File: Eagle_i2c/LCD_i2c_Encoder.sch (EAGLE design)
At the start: 8 parts, among them J1 455-1750-1-ND, U1 ARDUINOR3-BPLACE

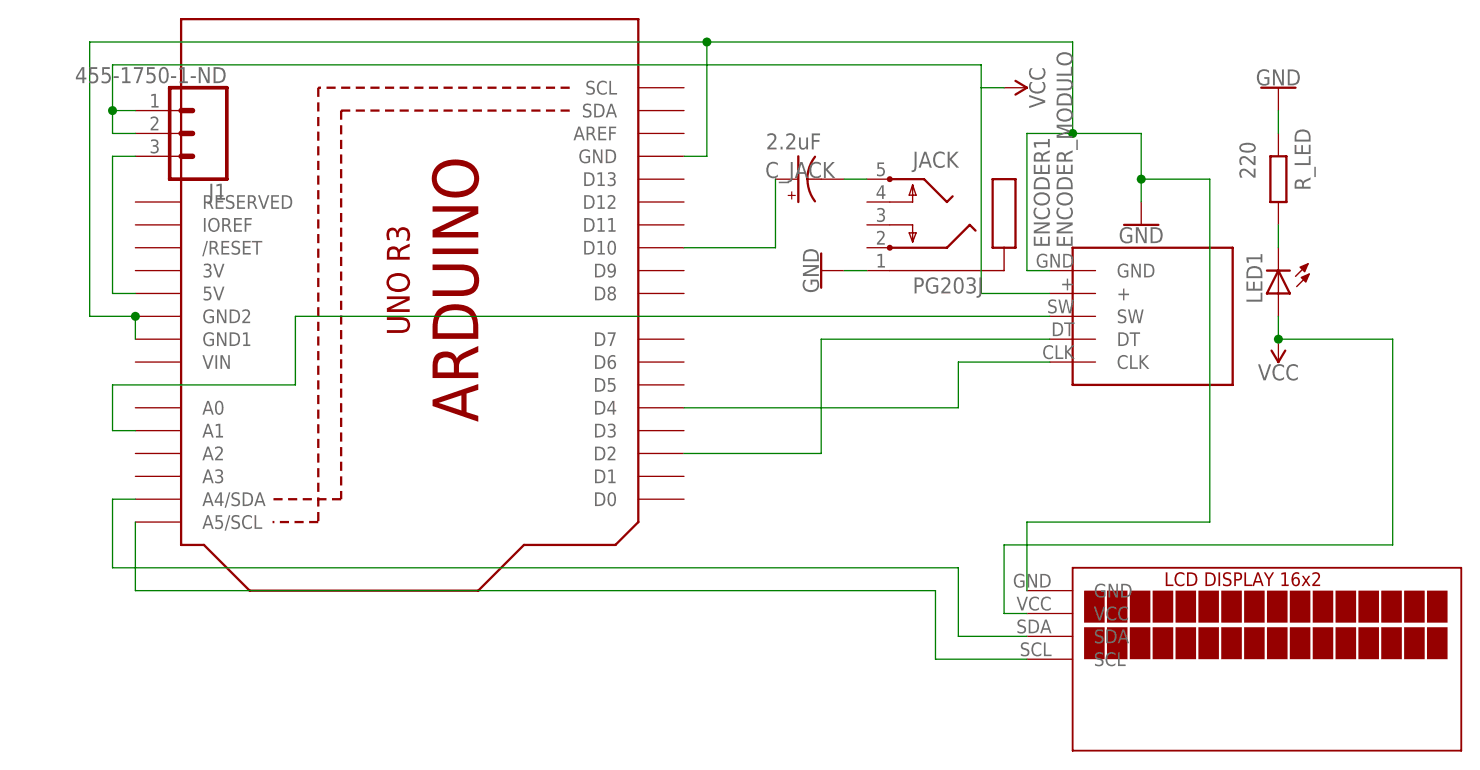
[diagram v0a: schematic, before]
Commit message: Version para imprimir ICAT, Gerbers incluidos
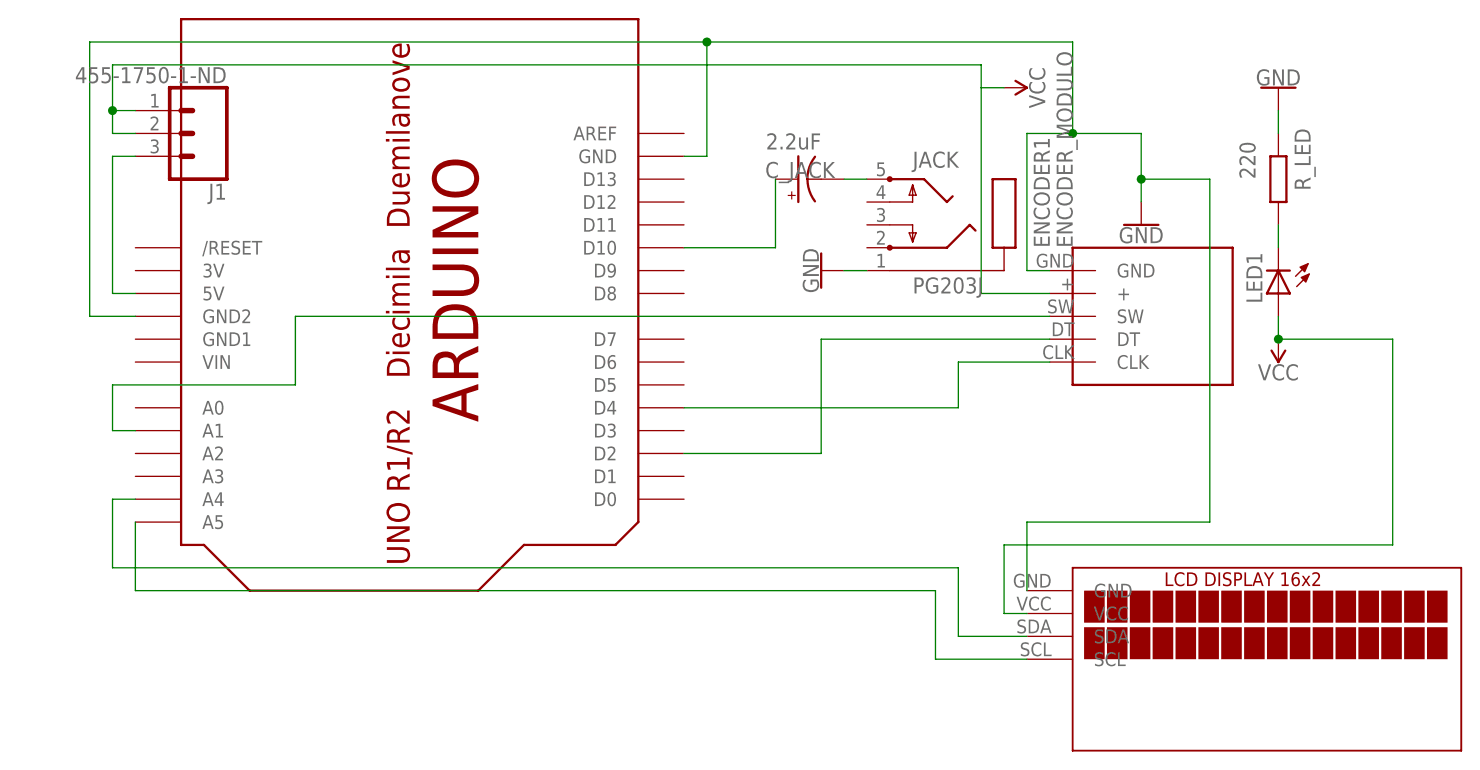
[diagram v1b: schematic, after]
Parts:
- removed U1: ARDUINOR3-BPLACE, adafruit:ARDUINOR3-BPLACE
- added U$1: ARDUINOUNO, Arduino_Espejo:ARDUINOUNO
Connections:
- net GND: now also U$1.GND, U$1.GND2; no longer U1.GND, U1.GND1, U1.GND2
- net N$1: now also U$1.D10; no longer U1.D10
- net N$17: now also U$1.D4; no longer U1.D4
- net N$18: now also U$1.D2; no longer U1.D2
- net N$3: now also U$1.A1; no longer U1.A1
- net N$5: now also U$1.5V; no longer U1.5V
- net N$8: now also U$1.A4; no longer U1.A4/SDA
- net N$9: now also U$1.A5; no longer U1.A5/SCL
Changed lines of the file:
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@@
 </variantdefs>
 <classes>
-<class number="0" name="default" width="0.3" drill="0.0127">
-<clearance class="0" value="0.3"/>
+<class number="0" name="default" width="0.3048" drill="0.3048">
+<clearance class="0" value="0.3048"/>
 </class>
 </classes>
@@
 <attribute name="CAPACITANCIA" value="2.2uF"/>
 </part>
-<part name="U1" library="adafruit" deviceset="ARDUINOR3" device="-BPLACE"/>
 <part name="SUPPLY1" library="SparkFun-PowerSymbols" deviceset="VCC" device=""/>
 <part name="SUPPLY2" library="SparkFun-PowerSymbols" deviceset="VCC" device=""/>
@@
 <part name="ENCODER1" library="ENCODER" deviceset="ENCODER_MODULO" device=""/>
 <part name="J1" library="SparkFun-Connectors" deviceset="CONN_03" device="" value="455-1750-1-ND"/>
+<part name="U$1" library="Arduino_Espejo" deviceset="ARDUINO" device="UNO"/>
 </parts>
 <sheets>
@@
 <attribute name="CAPACITANCIA" x="71.12" y="81.28" size="1.778" layer="96" rot="R180"/>
 </instance>
-<instance part="U1" gate="G$1" x="25.4" y="60.96" smashed="yes" rot="R270"/>
 <instance part="SUPPLY1" gate="G$1" x="91.44" y="86.36" smashed="yes" rot="R270">
 <attribute name="VALUE" x="94.234" y="86.36" size="1.778" layer="96" rot="R270" align="bottom-center"/>
@@
 <attribute name="NAME" x="5.08" y="75.692" size="1.778" layer="95" font="vector" rot="R180"/>
 </instance>
+<instance part="U$1" gate="G$1" x="27.94" y="71.12" smashed="yes" rot="R270"/>
 </instances>
 <busses>
@@
 <wire x1="99.06" y1="81.28" x2="106.68" y2="81.28" width="0.1524" layer="91"/>
 <wire x1="106.68" y1="81.28" x2="106.68" y2="76.2" width="0.1524" layer="91"/>
-<pinref part="U1" gate="G$1" pin="GND2"/>
 <wire x1="106.68" y1="76.2" x2="106.68" y2="73.66" width="0.1524" layer="91"/>
-<wire x1="-5.08" y1="60.96" x2="-10.16" y2="60.96" width="0.1524" layer="91"/>
 <wire x1="-10.16" y1="60.96" x2="-10.16" y2="91.44" width="0.1524" layer="91"/>
 <wire x1="-10.16" y1="91.44" x2="58.42" y2="91.44" width="0.1524" layer="91"/>
@@
 <wire x1="99.06" y1="91.44" x2="99.06" y2="81.28" width="0.1524" layer="91"/>
 <junction x="99.06" y="81.28"/>
-<pinref part="U1" gate="G$1" pin="GND1"/>
-<wire x1="-5.08" y1="58.42" x2="-5.08" y2="60.96" width="0.1524" layer="91"/>
-<junction x="-5.08" y="60.96"/>
-<pinref part="U1" gate="G$1" pin="GND"/>
-<wire x1="55.88" y1="78.74" x2="58.42" y2="78.74" width="0.1524" layer="91"/>
 <wire x1="58.42" y1="78.74" x2="58.42" y2="91.44" width="0.1524" layer="91"/>
 <junction x="58.42" y="91.44"/>
@@
 <pinref part="ENCODER1" gate="G$1" pin="GND"/>
 <wire x1="93.98" y1="66.04" x2="96.52" y2="66.04" width="0.1524" layer="91"/>
+<wire x1="-10.16" y1="60.96" x2="-5.08" y2="60.96" width="0.1524" layer="91"/>
+<wire x1="55.88" y1="78.74" x2="58.42" y2="78.74" width="0.1524" layer="91"/>
+<pinref part="U$1" gate="G$1" pin="GND"/>
+<pinref part="U$1" gate="G$1" pin="GND2"/>
 </segment>
 <segment>
@@
 <segment>
 <wire x1="86.36" y1="55.88" x2="86.36" y2="50.8" width="0.1524" layer="91"/>
-<pinref part="U1" gate="G$1" pin="D4"/>
-<wire x1="55.88" y1="50.8" x2="86.36" y2="50.8" width="0.1524" layer="91"/>
 <wire x1="86.36" y1="55.88" x2="96.52" y2="55.88" width="0.1524" layer="91"/>
 <pinref part="ENCODER1" gate="G$1" pin="CLK"/>
+<wire x1="86.36" y1="50.8" x2="55.88" y2="50.8" width="0.1524" layer="91"/>
+<pinref part="U$1" gate="G$1" pin="D4"/>
 </segment>
 </net>
@@
 <wire x1="71.12" y1="45.72" x2="71.12" y2="58.42" width="0.1524" layer="91"/>
 <wire x1="71.12" y1="58.42" x2="96.52" y2="58.42" width="0.1524" layer="91"/>
-<pinref part="U1" gate="G$1" pin="D2"/>
-<wire x1="55.88" y1="45.72" x2="71.12" y2="45.72" width="0.1524" layer="91"/>
 <pinref part="ENCODER1" gate="G$1" pin="DT"/>
+<wire x1="71.12" y1="45.72" x2="55.88" y2="45.72" width="0.1524" layer="91"/>
+<pinref part="U$1" gate="G$1" pin="D2"/>
 </segment>
 </net>
@@
 <segment>
 <wire x1="96.52" y1="60.96" x2="12.7" y2="60.96" width="0.1524" layer="91"/>
-<pinref part="U1" gate="G$1" pin="A1"/>
-<wire x1="-5.08" y1="48.26" x2="-7.62" y2="48.26" width="0.1524" layer="91"/>
 <wire x1="-7.62" y1="48.26" x2="-7.62" y2="53.34" width="0.1524" layer="91"/>
 <wire x1="-7.62" y1="53.34" x2="12.7" y2="53.34" width="0.1524" layer="91"/>
 <wire x1="12.7" y1="53.34" x2="12.7" y2="60.96" width="0.1524" layer="91"/>
 <pinref part="ENCODER1" gate="G$1" pin="SW"/>
+<wire x1="-5.08" y1="48.26" x2="-7.62" y2="48.26" width="0.1524" layer="91"/>
+<pinref part="U$1" gate="G$1" pin="A1"/>
 </segment>
 </net>
@@
 <pinref part="C_JACK" gate="G$1" pin="+"/>
 <wire x1="66.04" y1="76.2" x2="66.04" y2="68.58" width="0.1524" layer="91"/>
-<pinref part="U1" gate="G$1" pin="D10"/>
-<wire x1="66.04" y1="68.58" x2="55.88" y2="68.58" width="0.1524" layer="91"/>
+<wire x1="55.88" y1="68.58" x2="66.04" y2="68.58" width="0.1524" layer="91"/>
+<pinref part="U$1" gate="G$1" pin="D10"/>
 </segment>
 </net>
 <net name="N$5" class="0">
 <segment>
-<pinref part="U1" gate="G$1" pin="5V"/>
-<wire x1="-7.62" y1="63.5" x2="-5.08" y2="63.5" width="0.1524" layer="91"/>
 <wire x1="-7.62" y1="63.5" x2="-7.62" y2="78.74" width="0.1524" layer="91"/>
 <pinref part="J1" gate="J$1" pin="3"/>
 <wire x1="-5.08" y1="78.74" x2="-7.62" y2="78.74" width="0.1524" layer="91"/>
+<wire x1="-7.62" y1="63.5" x2="-5.08" y2="63.5" width="0.1524" layer="91"/>
+<pinref part="U$1" gate="G$1" pin="5V"/>
 </segment>
 </net>
@@
 <wire x1="86.36" y1="33.02" x2="-7.62" y2="33.02" width="0.1524" layer="91"/>
 <wire x1="-7.62" y1="33.02" x2="-7.62" y2="40.64" width="0.1524" layer="91"/>
-<pinref part="U1" gate="G$1" pin="A4/SDA"/>
-<wire x1="-7.62" y1="40.64" x2="-5.08" y2="40.64" width="0.1524" layer="91"/>
 <pinref part="LCD1" gate="G$1" pin="SDA"/>
 <wire x1="86.36" y1="33.02" x2="86.36" y2="25.4" width="0.1524" layer="91"/>
 <wire x1="86.36" y1="25.4" x2="93.98" y2="25.4" width="0.1524" layer="91"/>
+<wire x1="-7.62" y1="40.64" x2="-5.08" y2="40.64" width="0.1524" layer="91"/>
+<pinref part="U$1" gate="G$1" pin="A4"/>
 </segment>
 </net>
 <net name="N$9" class="0">
 <segment>
-<pinref part="U1" gate="G$1" pin="A5/SCL"/>
 <wire x1="83.82" y1="30.48" x2="-5.08" y2="30.48" width="0.1524" layer="91"/>
-<wire x1="-5.08" y1="30.48" x2="-5.08" y2="38.1" width="0.1524" layer="91"/>
 <pinref part="LCD1" gate="G$1" pin="SCL"/>
 <wire x1="83.82" y1="30.48" x2="83.82" y2="22.86" width="0.1524" layer="91"/>
 <wire x1="83.82" y1="22.86" x2="93.98" y2="22.86" width="0.1524" layer="91"/>
-</segment>
-</net>
+<wire x1="-5.08" y1="30.48" x2="-5.08" y2="38.1" width="0.1524" layer="91"/>
+<pinref part="U$1" gate="G$1" pin="A5"/>
+</segment>
+</net>
